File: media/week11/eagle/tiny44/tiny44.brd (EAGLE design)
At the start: 35 x 29.7 mm, 10 parts, among them IC1 ATTINY44-SSU, X1 22-23-2041, X3 22-23-2041

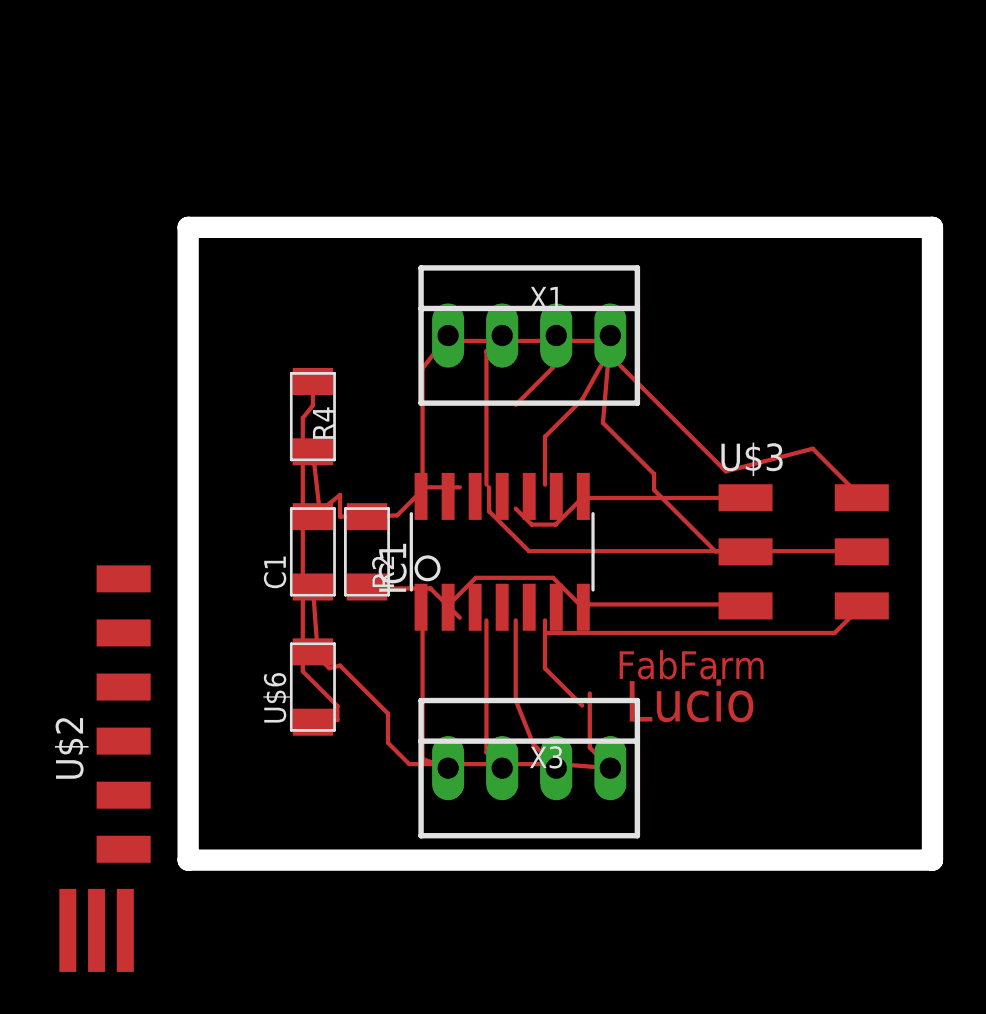
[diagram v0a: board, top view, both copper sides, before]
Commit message: week11 and start week16
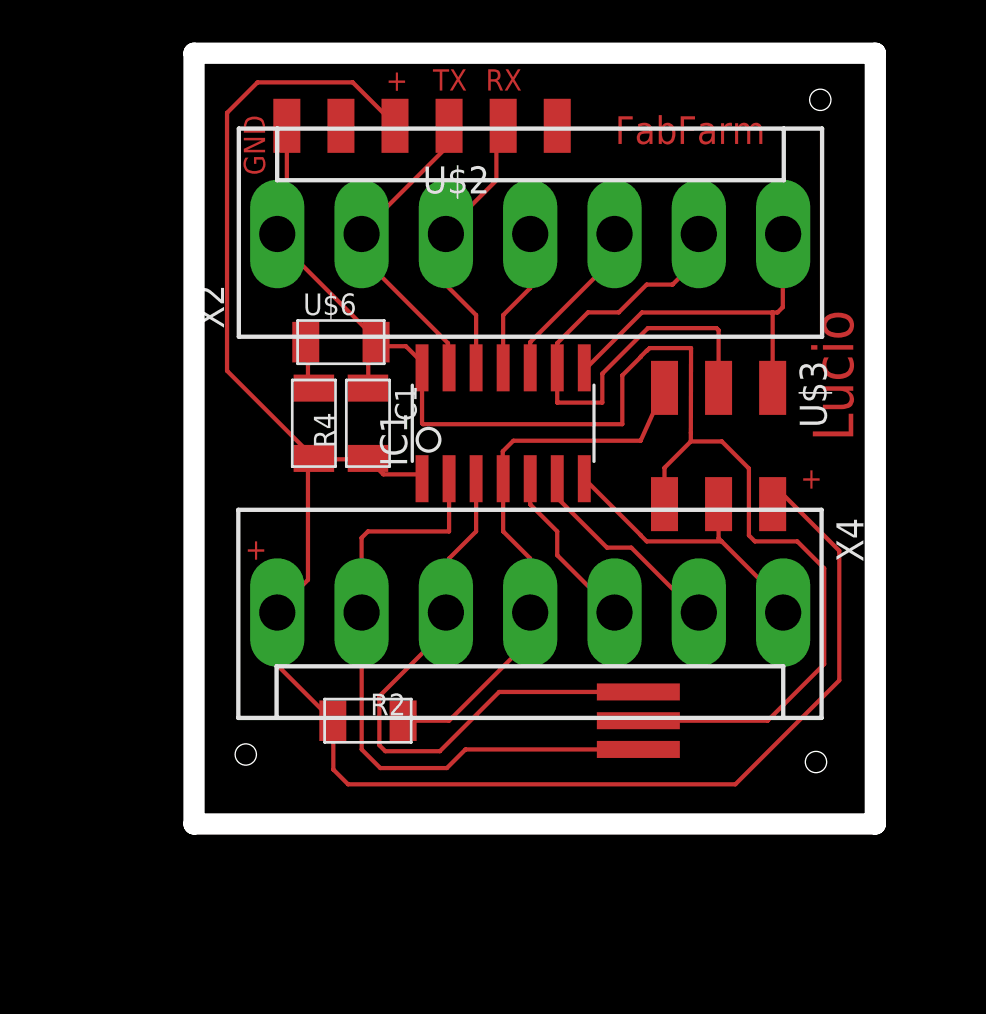
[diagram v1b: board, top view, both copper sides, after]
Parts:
- removed X1, X3: 22-23-2041, con-molex:22-23-2041
- added X2, X4: (no value), con-molex:KK-156-7
- moved U$2 31.0 mm to (11.5, 34.0), turned to 90 degrees
- moved U$1 27.3 mm to (21.6, 6.04), turned to 90 degrees
- moved U$6 16.3 mm to (7.67, 23.8), turned to 0 degrees
- moved R2 7.93 mm to (8.94, 6.04), turned to 180 degrees
- moved C1 6.57 mm to (8.94, 20.0), turned to 270 degrees
- moved U$3 6.41 mm to (25.4, 19.1), turned to 270 degrees
- moved IC1 6.04 mm to (15.3, 20.0)
- moved R4 0.31 mm to (6.40, 20.0)
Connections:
- removed net N$10: IC1.11
- removed net N$2: IC1.5
- removed net N$3: IC1.3, U$1.3
- removed net N$4: IC1.2, U$1.1
- removed net N$5: IC1.6
- removed net N$9: IC1.10
- removed net PT1: X3.3
- removed net PT2: X3.2
- new net 10: IC1.2, U$1.1, X4.6
- new net 8: IC1.5, X4.3
- new net 9: IC1.3, U$1.3, X4.5
- new net A2: IC1.11, X2.4
- new net A3: IC1.10, X2.5
- new net A7: IC1.6, X4.2
- net GND: now also X2.1; no longer X3.4
- net MISO: now also X2.7; no longer X1.3
- net MOSI: now also X4.1; no longer X1.4
- net RST: now also X4.4; no longer X3.1
- net RX: now also X2.3
- net SCK: now also X2.6; no longer X1.2
- net TX: now also X2.2
- net VCC: now also X4.7; no longer X1.1
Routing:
- net VCC: track 42.5 -> 85.9 mm
- net 10: track 0.00 -> 30.4 mm
- net 9: track 0.00 -> 27.8 mm
- net GND: track 44.2 -> 68.2 mm
- net PB2: track 17.9 -> 2.33 mm
- net TX: track 0.00 -> 14.9 mm
- net RX: track 0.00 -> 13.3 mm
- net MOSI: track 27.3 -> 14.0 mm
- net A7: track 0.00 -> 9.74 mm
- net A3: track 0.00 -> 7.93 mm
- net 8: track 0.00 -> 7.93 mm
- net PT1: track 7.53 -> 0.00 mm
- net PT2: track 7.25 -> 0.00 mm
- net A2: track 0.00 -> 6.81 mm
- net SCK: track 21.3 -> 24.8 mm
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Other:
- board size 35 x 29.7 mm -> 32 x 36.2 mm
- board text added: "+"
- board text added: "GND"
- board text added: "RX"
- board text added: "TX"
